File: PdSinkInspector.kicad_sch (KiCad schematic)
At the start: 57 parts, among them IC2 STUSB4700YQTR, J1 USB_C_Receptacle, J2 USB_C_Receptacle, Q1 AO3401A, Q2 AO3401A, Q3 AO3401A, SW1 SW_MEC_5E, SW2 SW_MEC_5E, U1 RP2040, U2 W25Q128JVS, U3 TPS63031DSK, Y2 Crystal_GND24

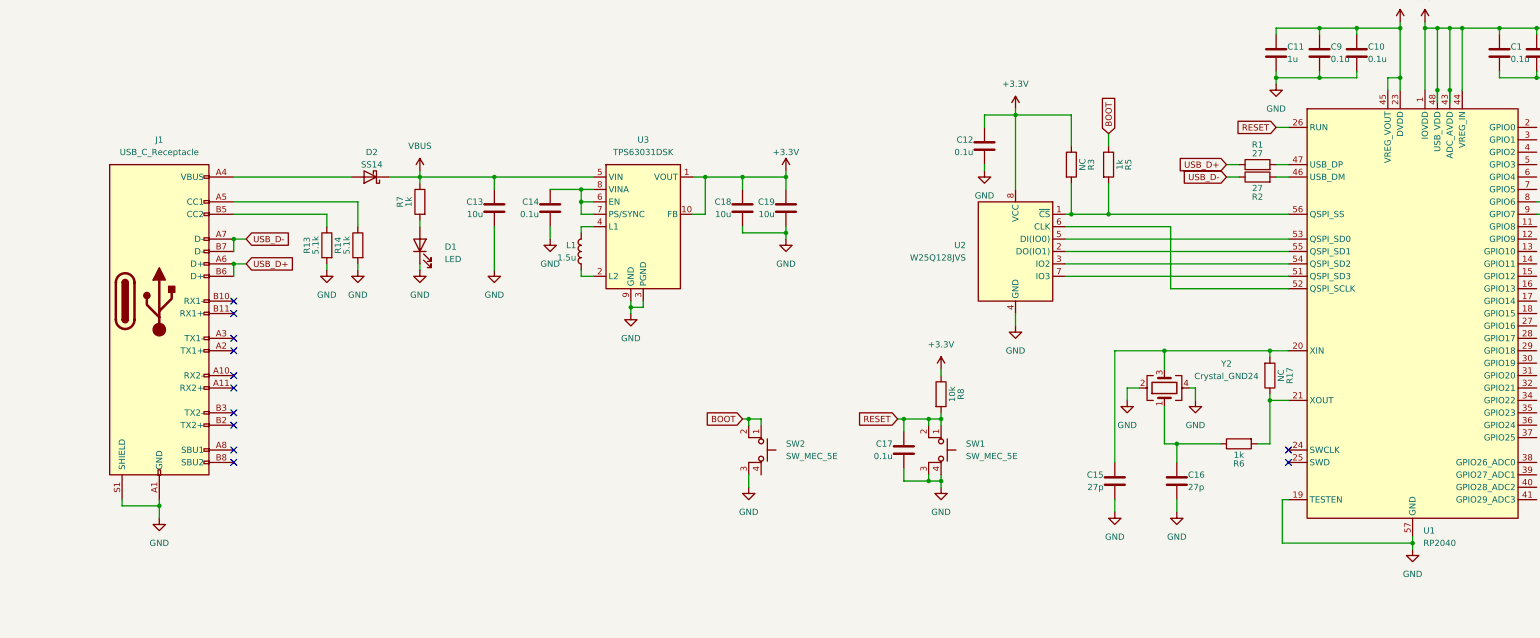
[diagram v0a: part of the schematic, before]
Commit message: [Update]基板配置してみた
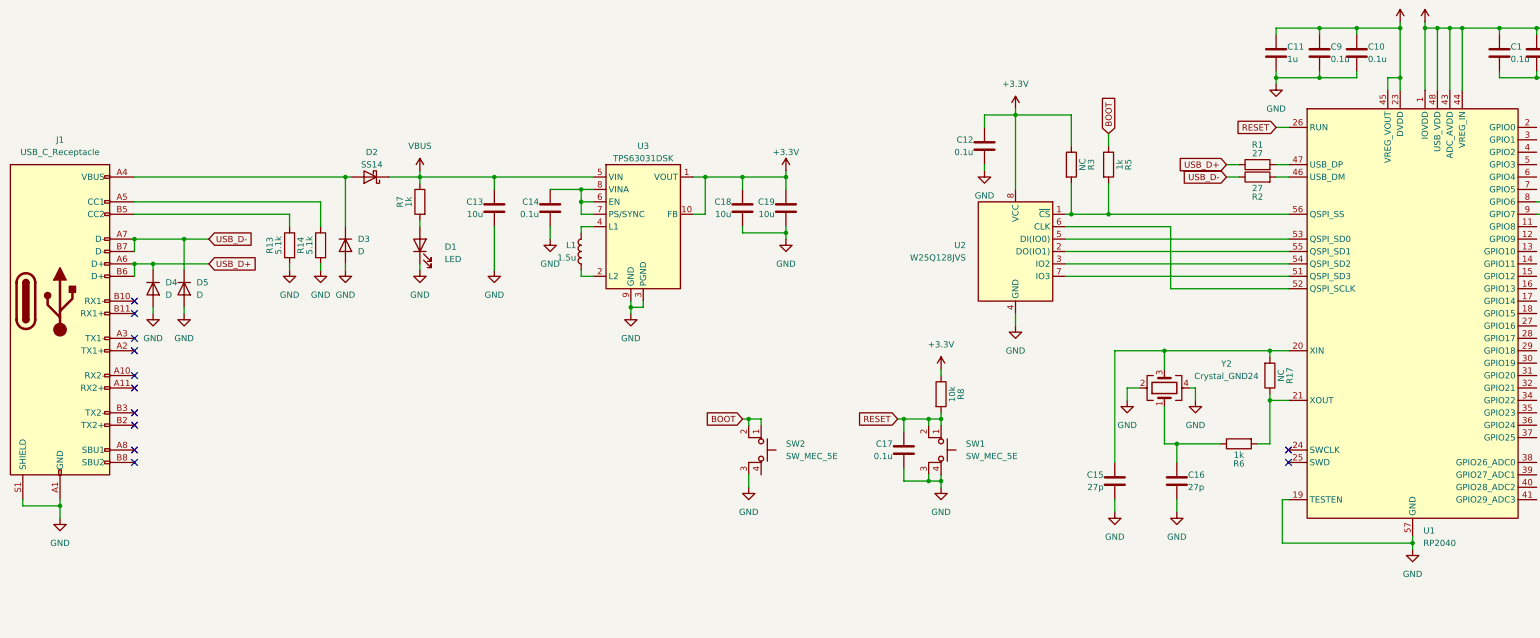
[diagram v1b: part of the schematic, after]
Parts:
- added D3, D4, D5: D, Diode_SMD:D_SOD-882, symbol Device:D
- Q1, Q2, Q3: BOM (none) -> C15127
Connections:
- net GND: now also D3.2 (A), D4.2 (A), D5.2 (A)
- net USB_D+: now also D4.1 (K)
- net USB_D-: now also D5.1 (K)
- net at D2.2 (A), J1.A4 (VBUS), J1.A9 (VBUS)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: now also D3.1 (K)
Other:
- moved on the sheet: J1, R13, R14

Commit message: [Update]基板配線開始+チップを0402に変更
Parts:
- removed J1, J2: USB_C_Receptacle, Connector_USB:USB_C_Receptacle_Molex_105450-0101, symbol Connector:USB_C_Receptacle
- added J1, J3: USB_C_Receptacle_USB2.0_16P, Connector_USB:USB_C_Receptacle_G-Switch_GT-USB-7010ASV, symbol Connector:USB_C_Receptacle_USB2.0_16P
- C1, C10, C12, C14, C17, C2, C3, C4, C5, C6, C7, C9: footprint Capacitor_SMD:C_0603_1608Metric -> Capacitor_SMD:C_0402_1005Metric; BOM C14663 -> C1525
- C11, C20, C21, C8: footprint Capacitor_SMD:C_0603_1608Metric -> Capacitor_SMD:C_0402_1005Metric; BOM C15849 -> C52923
- C13, C18, C19: footprint Capacitor_SMD:C_0603_1608Metric -> Capacitor_SMD:C_0402_1005Metric; BOM C14663 -> C15525
- C15, C16: footprint Capacitor_SMD:C_0603_1608Metric -> Capacitor_SMD:C_0402_1005Metric; BOM C107045 -> C1557
- R1, R2: footprint Resistor_SMD:R_0603_1608Metric -> Resistor_SMD:R_0402_1005Metric; BOM C4177 -> C25100
- R10: footprint Resistor_SMD:R_0603_1608Metric -> Resistor_SMD:R_0402_1005Metric; BOM C4177 -> C25879
- R11, R12, R8, R9: footprint Resistor_SMD:R_0603_1608Metric -> Resistor_SMD:R_0402_1005Metric; BOM C25804 -> C25744
- R13, R14: footprint Resistor_SMD:R_0603_1608Metric -> Resistor_SMD:R_0402_1005Metric; BOM C23186 -> C25905
- R15, R16: footprint Resistor_SMD:R_0603_1608Metric -> Resistor_SMD:R_0402_1005Metric; BOM C21190 -> C25900
- R4: footprint Resistor_SMD:R_0603_1608Metric -> Resistor_SMD:R_0402_1005Metric; BOM C4177 -> C25741
- R5, R6, R7: footprint Resistor_SMD:R_0603_1608Metric -> Resistor_SMD:R_0402_1005Metric; BOM C21190 -> C11702
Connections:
- net GND: now also J1.A1 (GND), J1.A12 (GND), J1.B1 (GND), J1.B12 (GND), J1.S1 (SHIELD), J3.A1 (GND), J3.A12 (GND), J3.B1 (GND), J3.B12 (GND), J3.S1 (SHIELD)
- net USB_D+: now also J3.A6 (D+), J3.B6 (D+)
- net USB_D-: now also J3.A7 (D-), J3.B7 (D-)
- net Vout: now also J1.A4 (VBUS), J1.A9 (VBUS), J1.B4 (VBUS), J1.B9 (VBUS)
- net at R14.1: now also J3.A5 (CC1)
- net at D2.2 (A), D3.1 (K): now also J3.A4 (VBUS), J3.A9 (VBUS), J3.B4 (VBUS), J3.B9 (VBUS)
- net at R13.1: now also J3.B5 (CC2)
- net at IC2.2 (CC1): now also J1.A5 (CC1)
- net at IC2.4 (CC2): now also J1.B5 (CC2)
- no-connect marks 35 -> 19
